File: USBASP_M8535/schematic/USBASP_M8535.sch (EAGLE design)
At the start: 74 parts, among them IC1 MEGA8535, J1 0, J2 0, Q1 12MHz, T1 BC847, T2 BC847, T3 BC847, T4 BC847, T5 BC847, X1 USB_B, X2 MCU_PROGRAMMING, X3 DEVICE_ISP, X4 DEVICE_JTAG_ISP

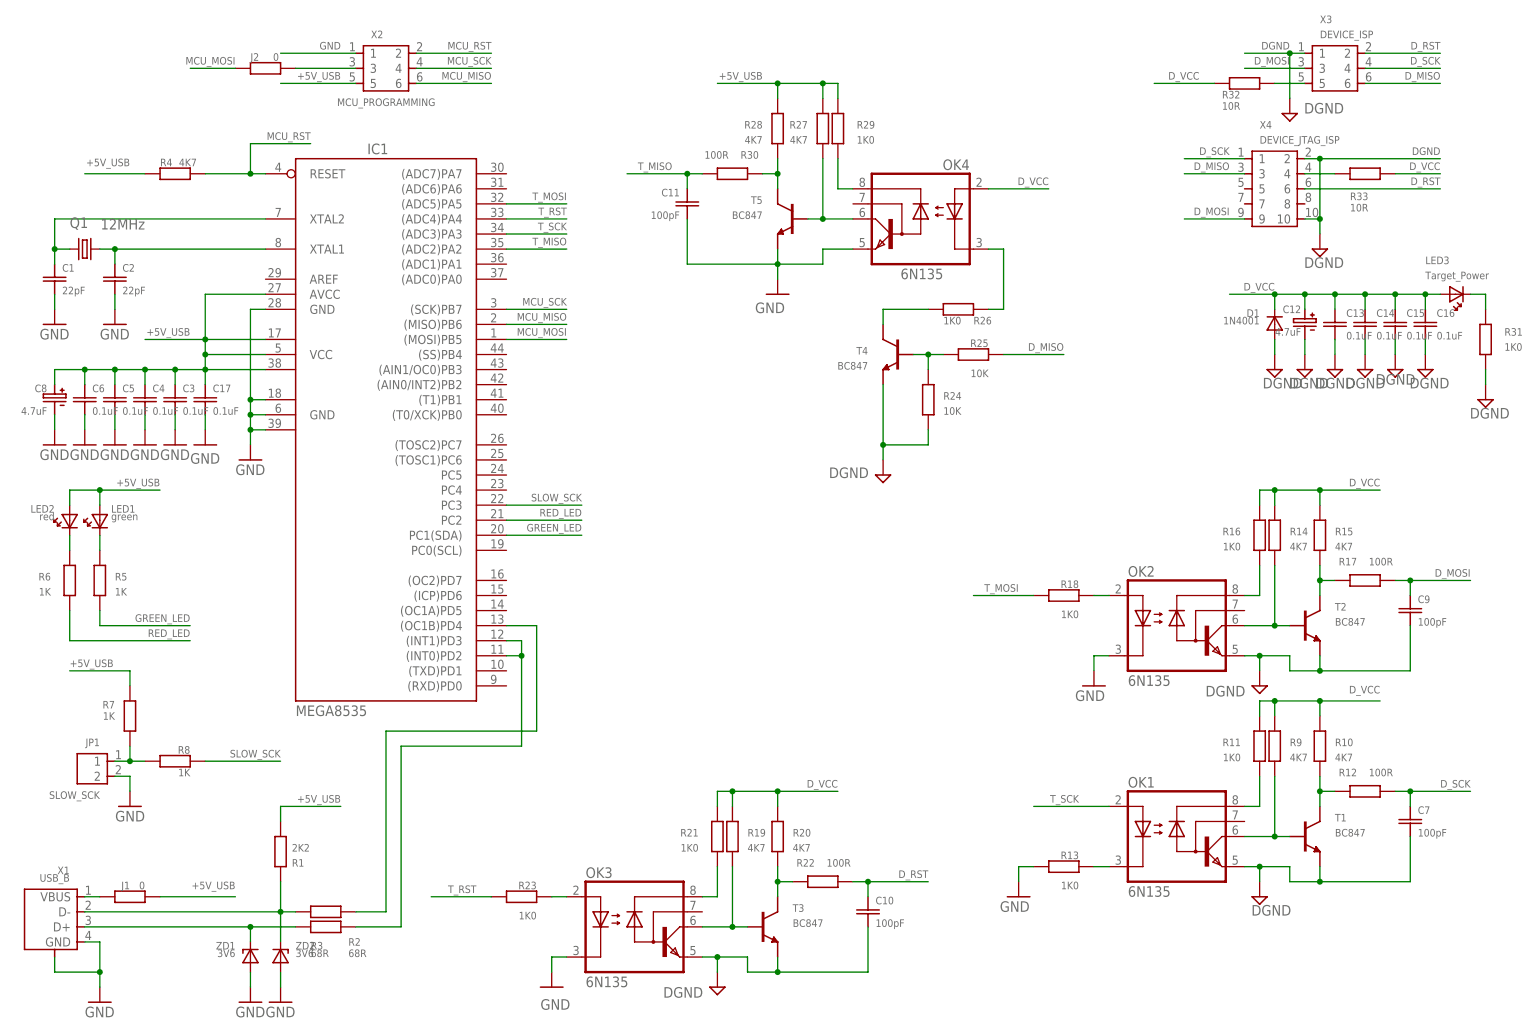
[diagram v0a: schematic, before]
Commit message: Some level converter values were changed for improve data transfer speed
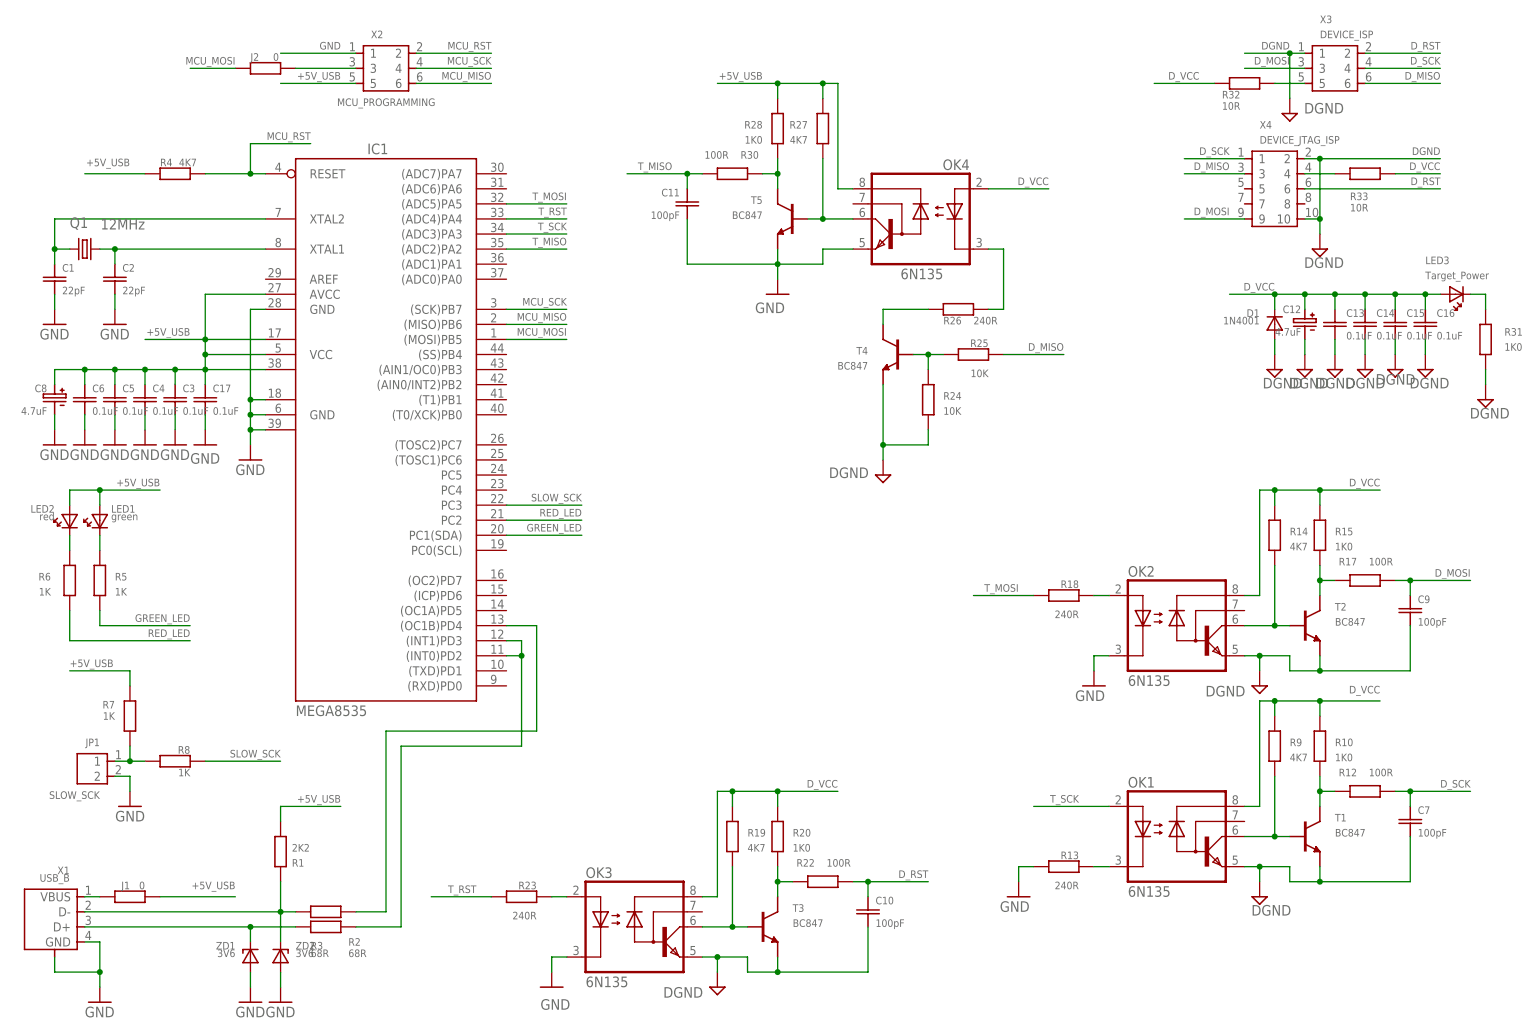
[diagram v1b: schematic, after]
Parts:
- removed R11, R16, R21, R29: 1K0, __MyCommonLib1:RSMD_0805
- R10, R15, R20, R28: value 4K7 -> 1K0
- R13, R18, R23, R26: value 1K0 -> 240R
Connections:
- removed net N$10: OK1.VCC, R11.PIN1
- removed net N$17: OK2.VCC, R16.PIN1
- removed net N$23: OK3.VCC, R21.PIN1
- removed net N$34: OK4.VCC, R29.PIN1
- net +5V_USB: now also OK4.VCC; no longer R29.PIN0
- net D_VCC: now also OK1.VCC, OK2.VCC, OK3.VCC; no longer R11.PIN0, R16.PIN0, R21.PIN0
